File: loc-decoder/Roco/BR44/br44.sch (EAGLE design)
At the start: 8 parts

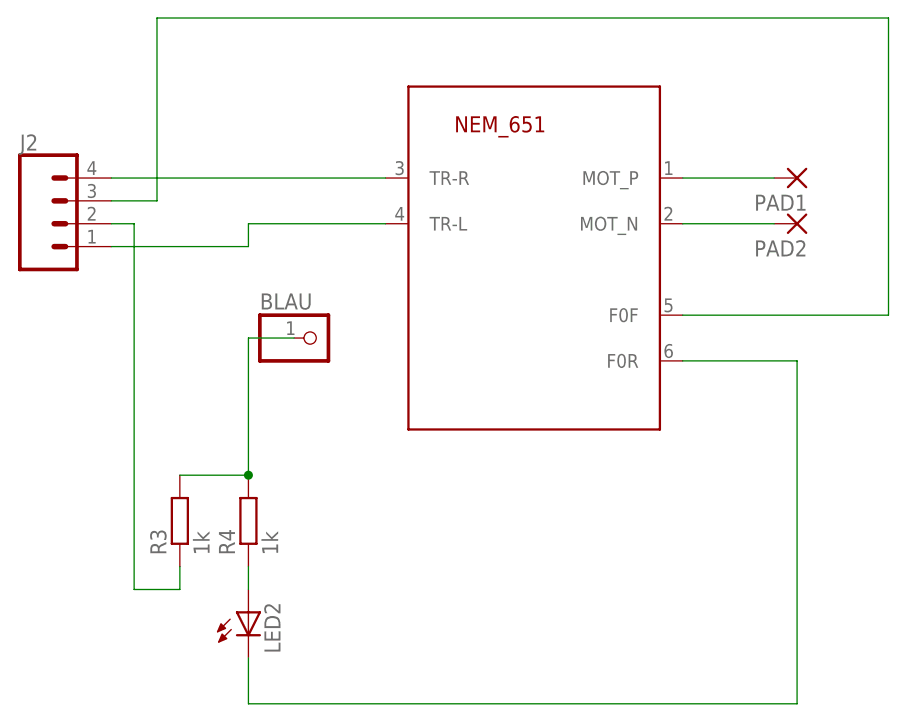
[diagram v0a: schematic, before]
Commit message: misc
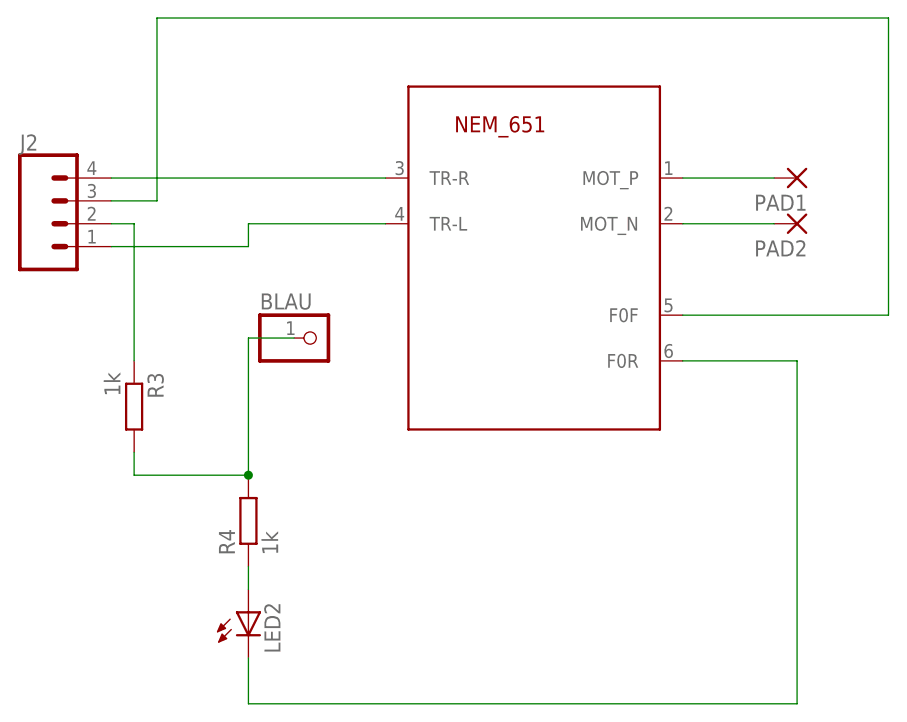
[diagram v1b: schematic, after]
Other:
- moved on the sheet: R3
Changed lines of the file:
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@@
 <?xml version="1.0" encoding="utf-8"?>
 <!DOCTYPE eagle SYSTEM "eagle.dtd">
-<eagle version="9.4.0">
+<eagle version="9.5.2">
 <drawing>
 <settings>
@@
 <attribute name="NAME" x="43.18" y="79.248" size="1.778" layer="95" font="vector"/>
 </instance>
-<instance part="R3" gate="G$1" x="60.96" y="38.1" smashed="yes" rot="R90">
-<attribute name="NAME" x="59.4614" y="34.29" size="1.778" layer="95" rot="R90"/>
-<attribute name="VALUE" x="64.262" y="34.29" size="1.778" layer="96" rot="R90"/>
+<instance part="R3" gate="G$1" x="55.88" y="50.8" smashed="yes" rot="R270">
+<attribute name="NAME" x="57.3786" y="54.61" size="1.778" layer="95" rot="R270"/>
+<attribute name="VALUE" x="52.578" y="54.61" size="1.778" layer="96" rot="R270"/>
 </instance>
 <instance part="R4" gate="G$1" x="68.58" y="38.1" smashed="yes" rot="R90">
@@
 <segment>
 <wire x1="68.58" y1="58.42" x2="68.58" y2="43.18" width="0.1524" layer="91"/>
-<wire x1="68.58" y1="43.18" x2="60.96" y2="43.18" width="0.1524" layer="91"/>
+<wire x1="68.58" y1="43.18" x2="55.88" y2="43.18" width="0.1524" layer="91"/>
+<wire x1="55.88" y1="43.18" x2="55.88" y2="45.72" width="0.1524" layer="91"/>
 <pinref part="R3" gate="G$1" pin="2"/>
 <pinref part="R4" gate="G$1" pin="2"/>
@@
 <net name="N$7" class="0">
 <segment>
-<wire x1="60.96" y1="33.02" x2="60.96" y2="30.48" width="0.1524" layer="91"/>
-<wire x1="60.96" y1="30.48" x2="55.88" y2="30.48" width="0.1524" layer="91"/>
-<wire x1="55.88" y1="30.48" x2="55.88" y2="71.12" width="0.1524" layer="91"/>
+<wire x1="55.88" y1="55.88" x2="55.88" y2="71.12" width="0.1524" layer="91"/>
 <pinref part="J2" gate="G$1" pin="2"/>
 <wire x1="55.88" y1="71.12" x2="53.34" y2="71.12" width="0.1524" layer="91"/>
